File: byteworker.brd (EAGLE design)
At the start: 32 x 32 mm, 65 parts, among them IC1 MCP1703, IC2 TJA1043, J2 AVRSPI-61.27, Q1 BSS138, Q2 BSS138, Q3 BSS138, Q5 BSS138, Q6 FDN5618P, X1 16 MHz, X2 bus connector

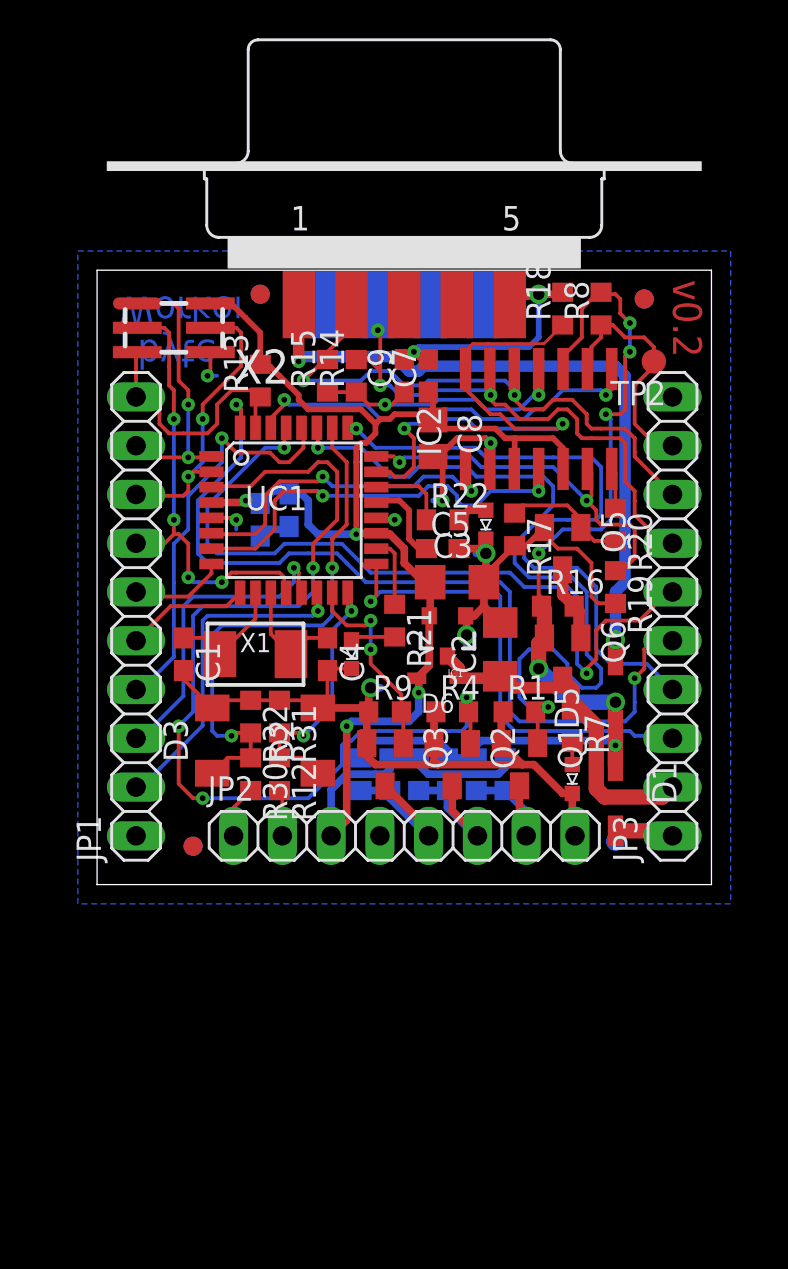
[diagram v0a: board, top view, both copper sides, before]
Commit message: Done routing
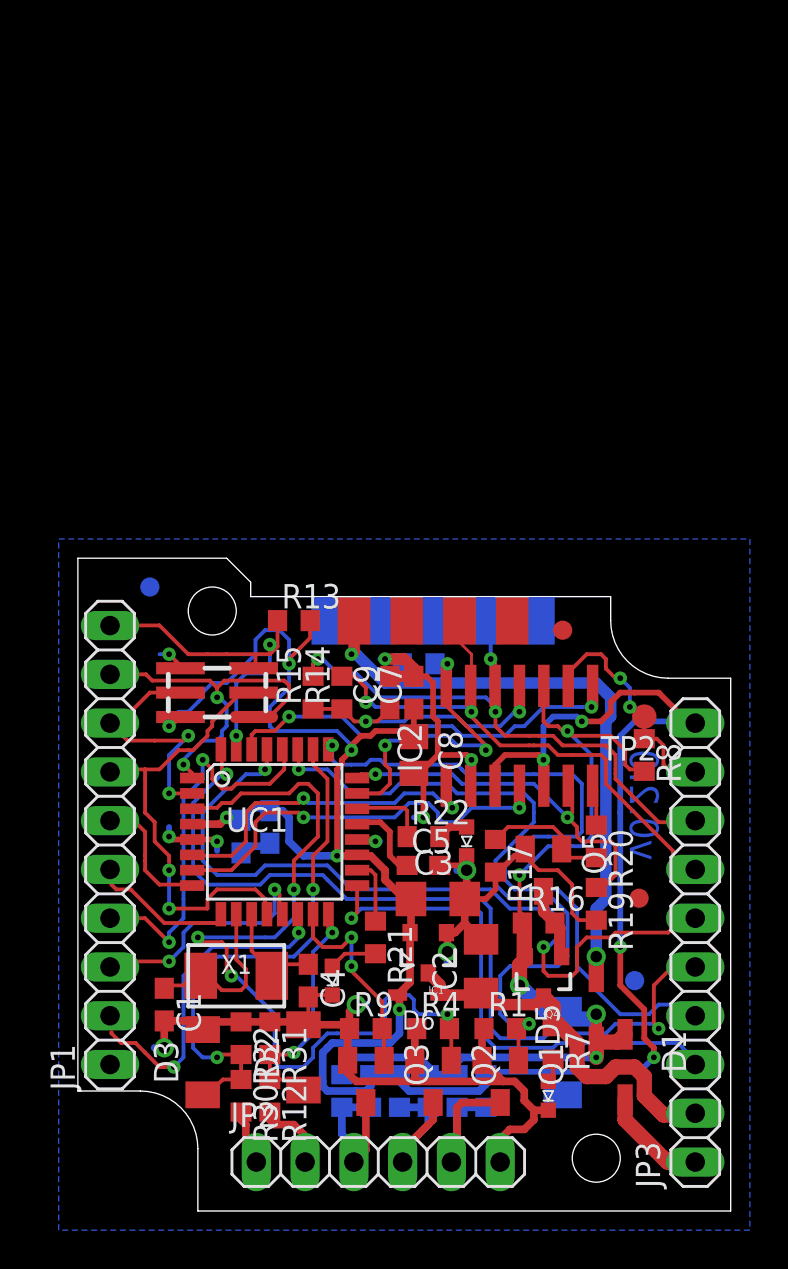
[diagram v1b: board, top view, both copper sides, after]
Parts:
- removed Q6: FDN5618P, bytewerk-fet:SOT23C
- removed U$3, U$7, U$8: (no value), bytewerk-symbol:FIDUCIAL_R
- removed X2: bus connector, con-subd:F09D
- added D4: 16V, bytewerk-diode:SOD-128
- added Q4: AP2321GN-HF-3TR, bytewerk-transistor:SOT23-3
- added X3: SUBD-H9, bytewerk-con:SUBD9
- C2: value 10u/25v -> 1u/25V
- C3: value 10u/10v -> 1u/10V
- JP2: device pinhead:1X08 -> pinhead:1X06
- LED1: value n.b.[yellow] -> green
- LED2: value n.b.[green] -> blue
- LED3: value n.b.[red] -> red
- moved U$2 37.1 mm to (12.2, -0.71)
- moved U$4 35.5 mm to (12.0, -5.00), flipped to the bottom
- moved U$6 27.6 mm to (-13.2, 15.5)
- moved R8 23.4 mm to (12.5, 6.75), turned to 270 degrees
- moved R18 20.0 mm to (0.75, 11.5), flipped to the bottom, turned to 0 degrees
- moved J2 19.1 mm to (-9.75, 10.0), turned to 90 degrees
- moved TP2 18.5 mm to (12.5, 8.75)
- moved C1 18.3 mm to (-12.5, -6.25)
- moved U$5 17.8 mm to (8.25, 13.2), flipped to the top
- moved JP2 17.0 mm to (-1.35, -14.4)
- moved JP3 17.0 mm to (15.2, -3.02)
- moved C4 17.0 mm to (-5.00, -5.00)
- moved LED1 17.0 mm to (-3.75, -5.00)
- moved R17 17.0 mm to (4.75, 1.50)
- moved Q5 16.8 mm to (7.25, 0.75)
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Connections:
- net +5V: now also JP3.10; no longer JP2.3
- net CANH: now also X3.7; no longer X2.7
- net CANL: now also X3.2; no longer X2.2
- net GND: now also D4.A, JP2.6, X3.3; no longer JP2.8, JP3.10, X2.5
- net N$6: now also Q4.1; no longer Q6.1
- net OUT0: now also JP2.5; no longer JP2.7
- net OUT1: now also JP2.4; no longer JP2.6
- net OUT2: now also JP2.3; no longer JP2.5
- net VIN_BUS: now also X3.9; no longer X2.1
- net VIN_RECT: now also D4.C, Q4.2; no longer Q6.2
- net VOUT_SW: now also Q4.3; no longer Q6.3
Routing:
- net +5V: track 80.3 -> 122.7 mm, vias 4 -> 10
- net !CAN_STB!: track 26.9 -> 15.8 mm, vias 2 -> 3
- net SS_A/OC1B: track 51.3 -> 43.6 mm
- net !RESET!: track 13.7 -> 18.9 mm, vias 0 -> 2
- net MISO_A/OC1A: track 14.4 -> 19.5 mm
- net VIN_BUS: track 35.7 -> 31.1 mm
- net PB6: track 40.9 -> 36.5 mm
- net D2A: track 34.2 -> 37.9 mm
- net PD5/ADC2: track 16.5 -> 12.9 mm, vias 1 -> 2
- net VIN_RECT: track 53.3 -> 50.0 mm, vias 7 -> 5
- net OUT0: track 7.07 -> 9.80 mm
- net N$1: track 6.23 -> 8.85 mm
- net VIN_EXT: track 3.08 -> 5.62 mm
- net PC4: track 24.8 -> 27.3 mm
- net VOUT_SW: track 18.2 -> 20.1 mm
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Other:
- board size 32 x 32 mm -> 34 x 34 mm
- board text added: "v0.2.0"
- board text removed: "byte- Worker"
- board text removed: "v0.2"
